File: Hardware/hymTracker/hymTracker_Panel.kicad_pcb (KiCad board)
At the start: 2 copper layers, 93.7 x 54.6 mm, 38 parts, among them J1 DB9_Female, Q1 2N7000, U1 MP1584_DCDC, U2 GY-NEO6MV2

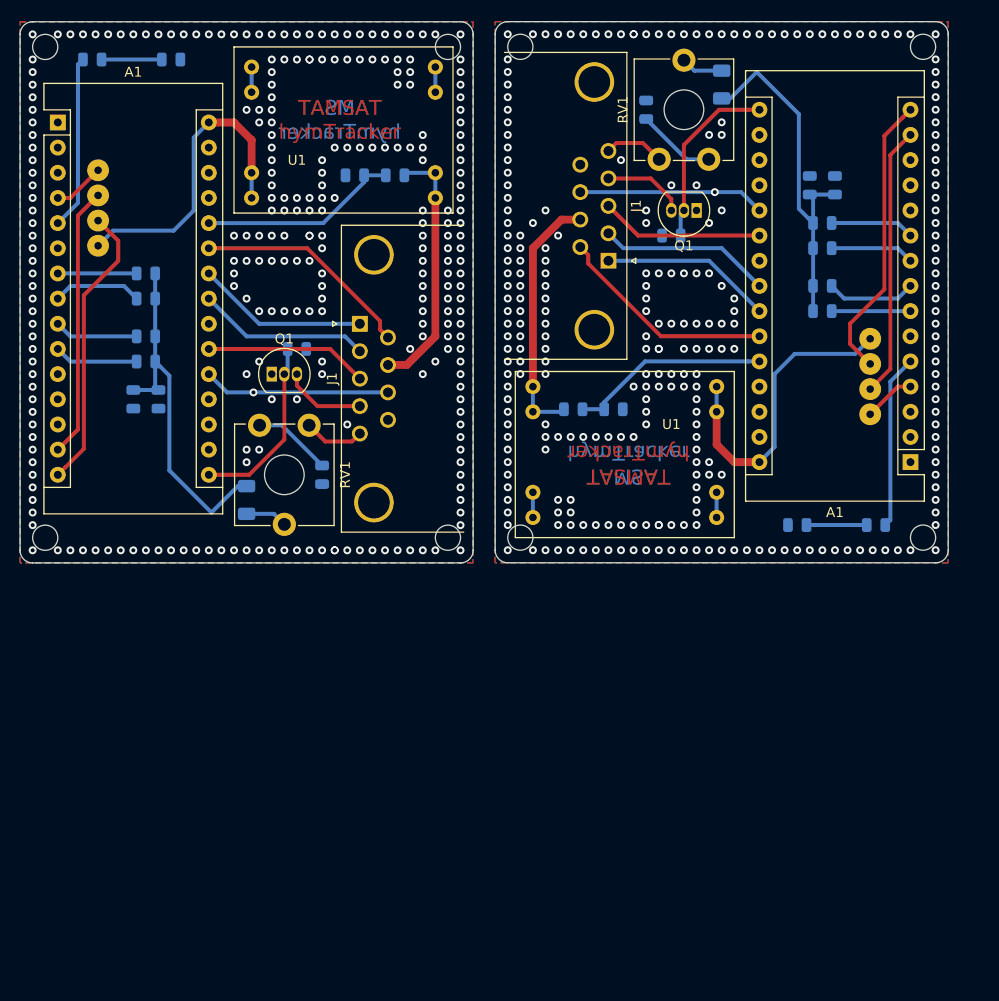
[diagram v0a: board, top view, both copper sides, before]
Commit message: panel.. callsign and RULER added
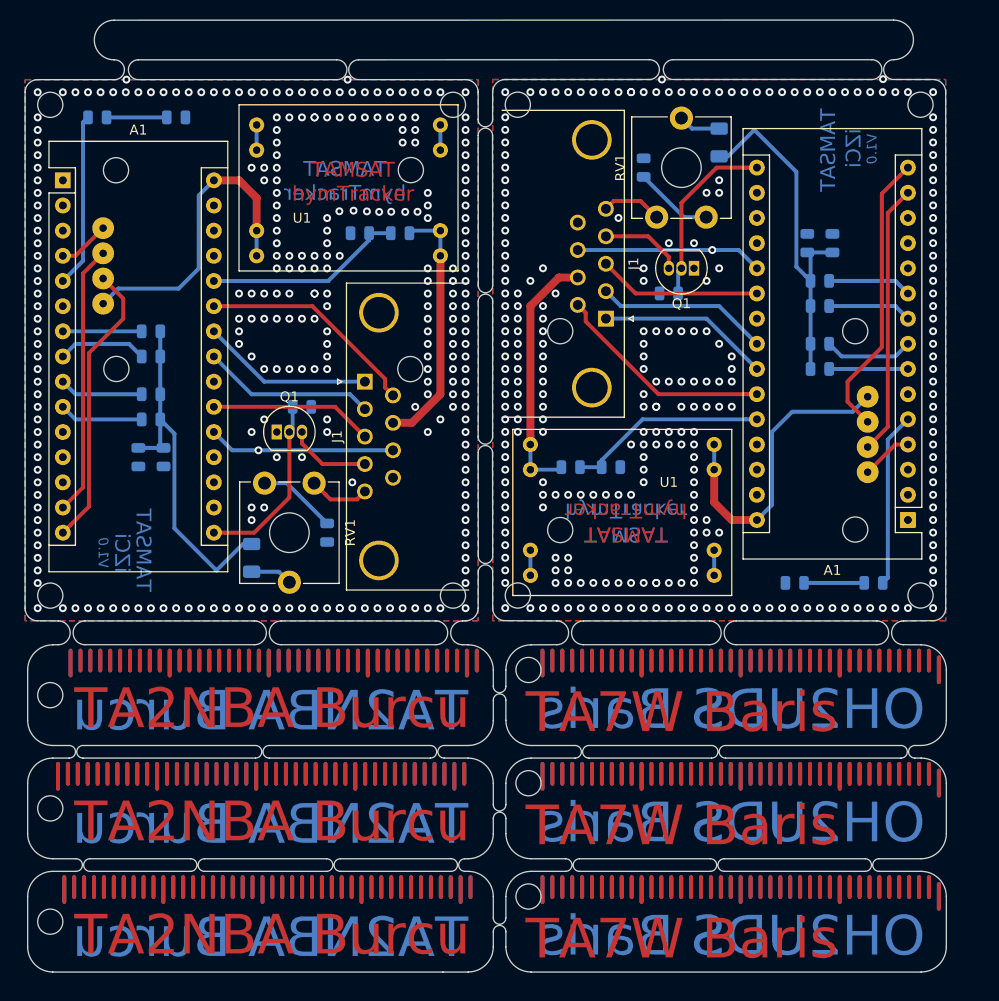
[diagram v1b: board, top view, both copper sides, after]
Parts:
- moved R7 5.86 mm to (41.7, 82.7)
- moved U1 5.86 mm to (63.2, 61.1)
- moved A1 5.86 mm to (32.8, 58.5)
- moved D1 5.86 mm to (44.2, 52.2)
- moved R10 5.86 mm to (59.4, 94.1)
- moved R2 5.86 mm to (62.7, 63.9)
- moved R3 5.86 mm to (36.2, 52.2)
- moved R4 5.86 mm to (41.7, 73.8)
- moved R5 5.86 mm to (41.7, 76.3)
- moved R6 5.86 mm to (41.7, 80.1)
- moved R8 5.86 mm to (56.9, 81.4)
- moved RV1 5.86 mm to (53.1, 89.1)
- moved C1 5.86 mm to (40.4, 86.5)
- moved C2 5.86 mm to (51.8, 96.6)
- moved J1 5.86 mm to (63.2, 78.9)
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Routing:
- net (no net): track 376.3 -> 1402.3 mm, vias 275 -> 279
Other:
- board size 93.7 x 54.6 mm -> 93 x 96.1 mm
- board text added: "OH2UDS Baris"
- board text added: "TA2NBA Burcu"
- board text added: "TA7W Baris"
- board text added: "TAMSAT"
- board text added: "V1.0"
- board text added: "iZCi"
